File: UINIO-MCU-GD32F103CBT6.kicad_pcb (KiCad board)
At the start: 2 copper layers, 68.4 x 20.3 mm, 41 parts, among them J1 Conn_01x24_Pin, J2 Conn_01x24_Pin, J3 Conn_01x04_Pin, SW1 BOOT1, SW2 NRST, SW3 BOOT0, U1 ME6211C33M5G-N, U2 GD32F103C8T6, Y1 32.768KHz, Y2 8MHz

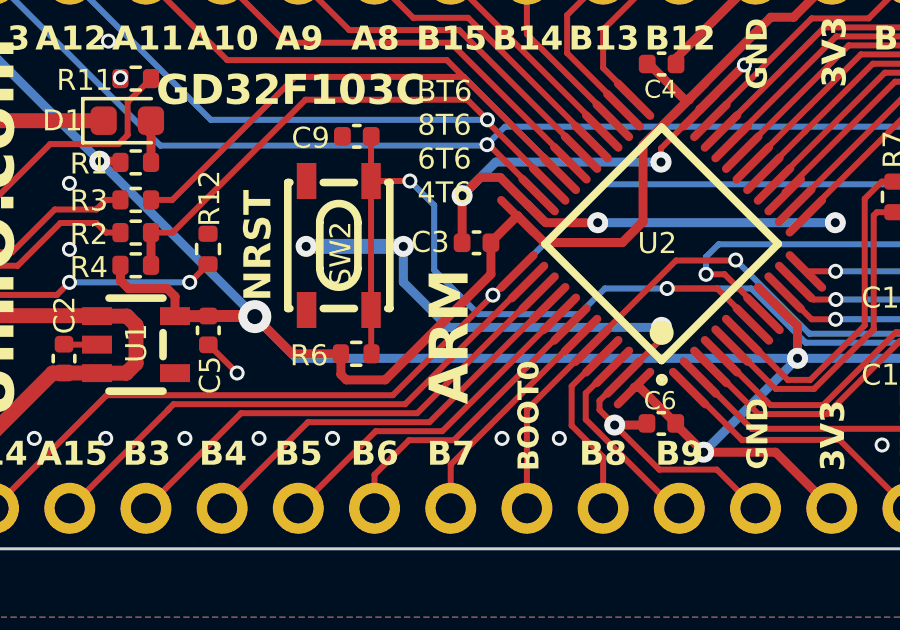
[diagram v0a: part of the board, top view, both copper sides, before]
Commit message: Release UINIO-MCU-GD32F103CBT6 version 3.1.2.
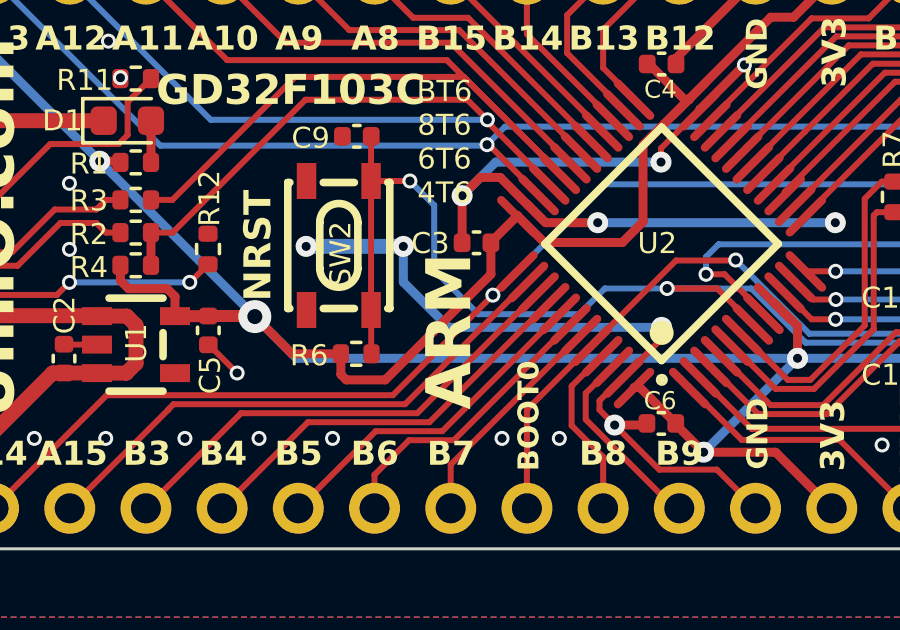
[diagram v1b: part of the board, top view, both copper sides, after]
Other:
- board text added: "Version 3.1.2"
- board text removed: "Version 3.1.1"
